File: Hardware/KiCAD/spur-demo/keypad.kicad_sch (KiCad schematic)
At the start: 40 parts, among them SW10 *, SW11 4, SW12 5, SW13 6, SW14 0, SW15 7, SW16 8, SW17 9, SW18 #, SW19 PTT, SW20 LEFT, SW21 RIGHT, SW22 SK0, SW3 MENU, SW4 UP, SW5 DOWN, SW6 EXIT, SW7 1, SW8 2, SW9 3

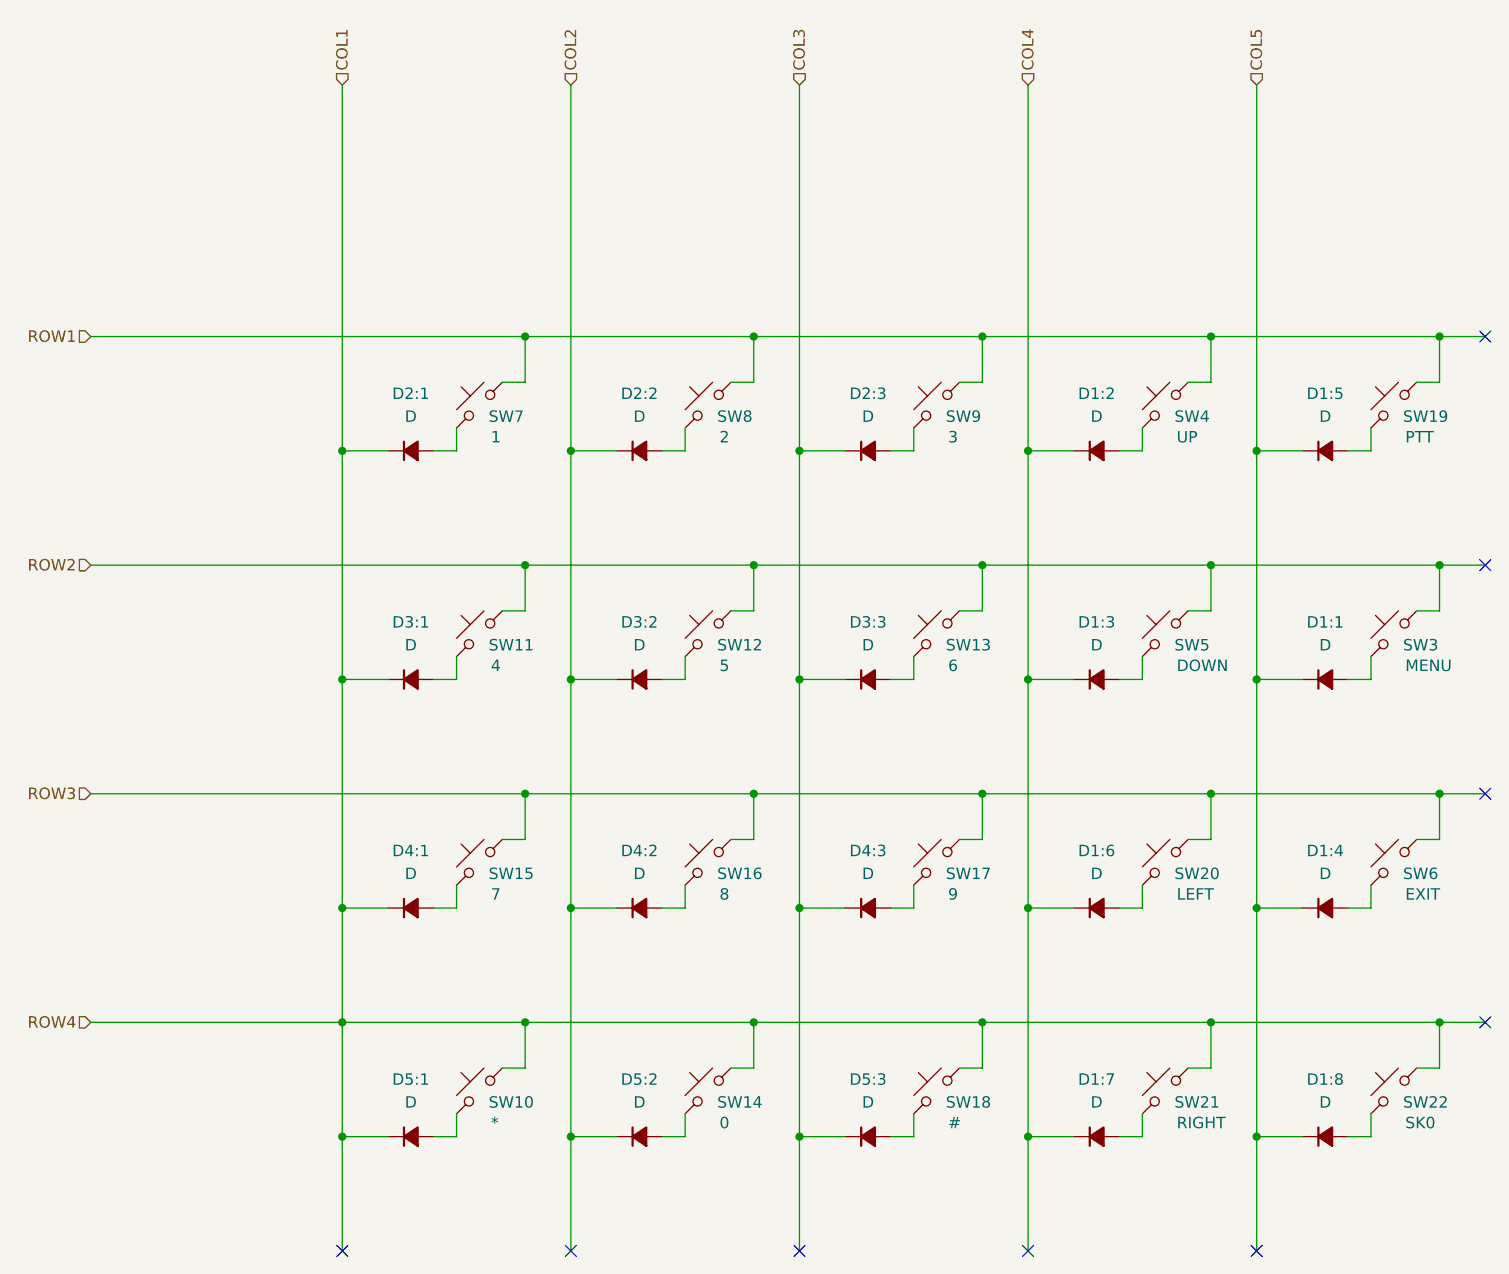
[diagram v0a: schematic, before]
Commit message: fix: remove node breaking col1 and row4 net resolution
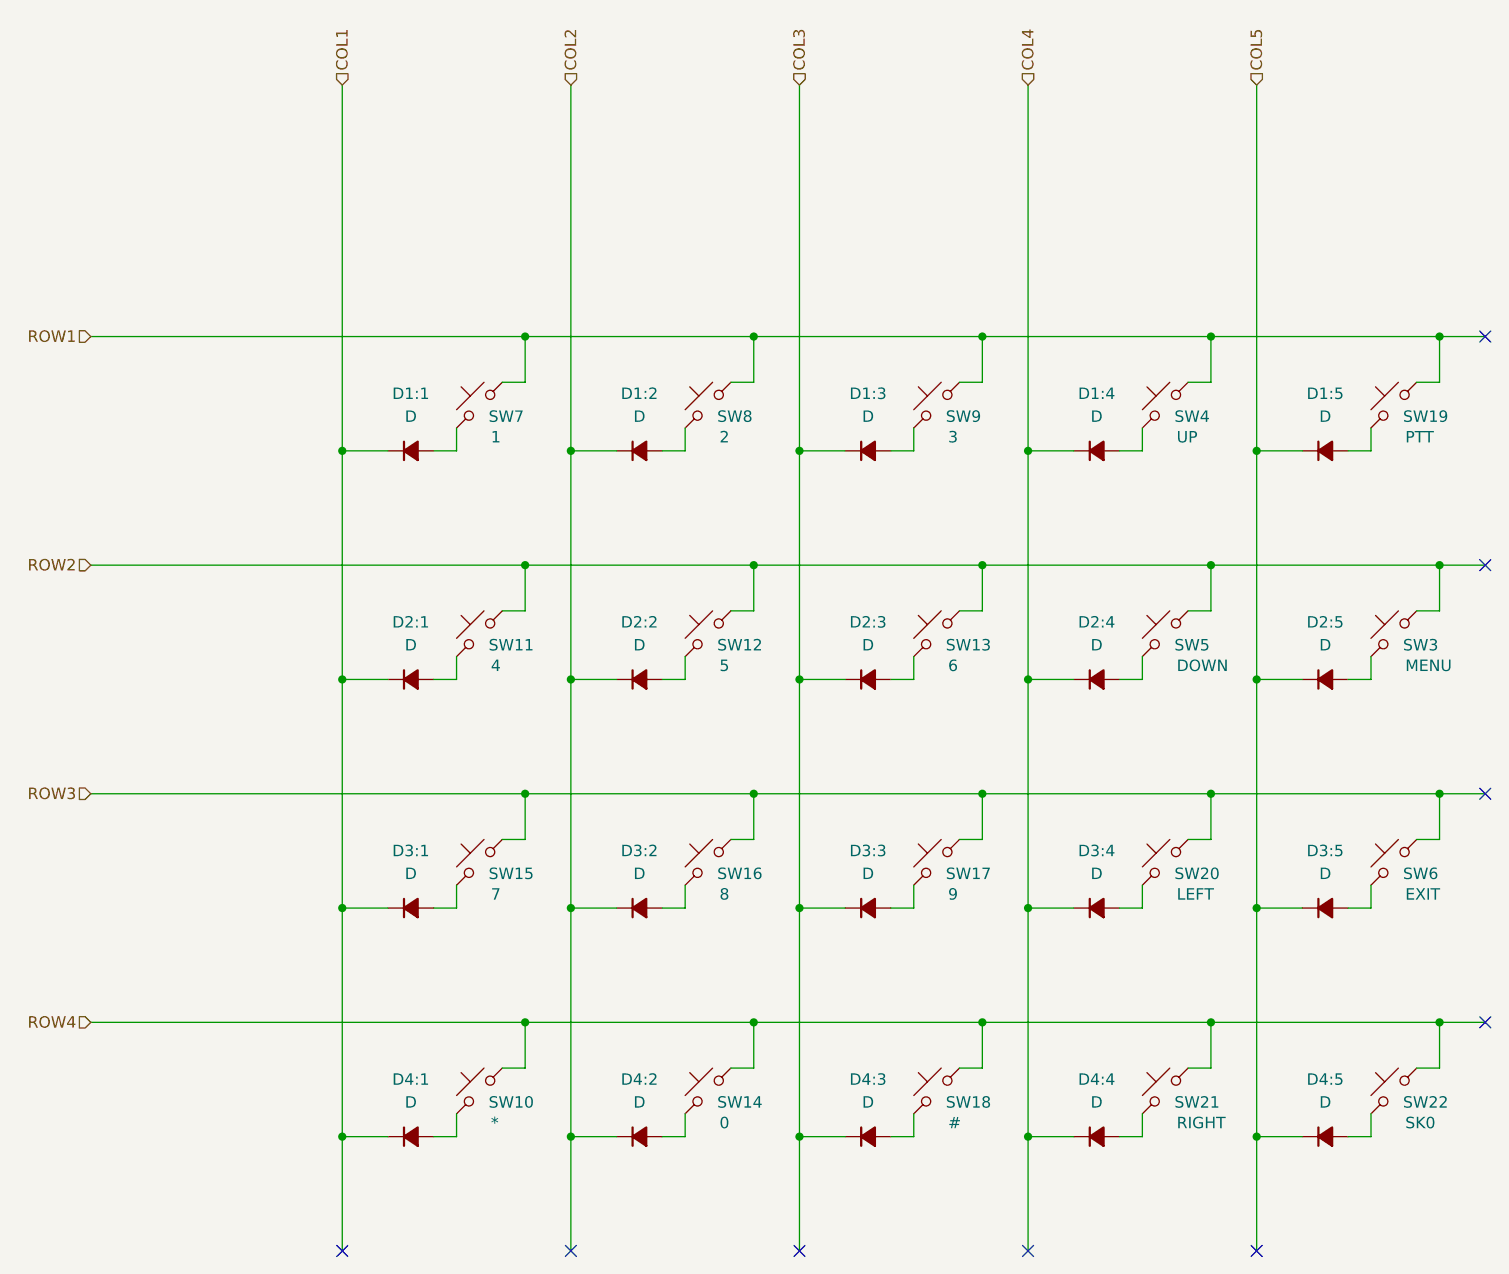
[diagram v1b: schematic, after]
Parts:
- renumbered D2:1 to D1:1, D2:2 to D1:2, D2:3 to D1:3, D1:2 to D1:4, D3:1 to D2:1, D3:2 to D2:2, D3:3 to D2:3, D1:3 to D2:4, D1:1 to D2:5, D4:1 to D3:1, D4:2 to D3:2, D4:3 to D3:3, D1:6 to D3:4, D1:4 to D3:5, D5:1 to D4:1, D5:2 to D4:2, D5:3 to D4:3, D1:7 to D4:4, D1:8 to D4:5
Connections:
- net COL1: no longer SW10.2, SW14.2, SW18.2, SW21.2, SW22.2
- new net ROW4: SW10.2, SW14.2, SW18.2, SW21.2, SW22.2
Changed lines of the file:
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@@
 	)
 	(junction
-		(at 76.2 135.89)
-		(diameter 0)
-		(color 0 0 0 0)
-	)
-	(junction
 		(at 127 123.19)
 		(diameter 0)
@@
 	(wire
 		(pts
-			(xy 76.2 123.19) (xy 76.2 135.89)
+			(xy 76.2 123.19) (xy 76.2 148.59)
 		)
 		(stroke
@@
 	(wire
 		(pts
-			(xy 48.26 135.89) (xy 76.2 135.89)
+			(xy 48.26 135.89) (xy 96.52 135.89)
 		)
 		(stroke
@@
 	(wire
 		(pts
-			(xy 76.2 135.89) (xy 76.2 148.59)
-		)
-		(stroke
-			(width 0)
-			(type default)
-		)
-	)
-	(wire
-		(pts
 			(xy 152.4 97.79) (xy 157.48 97.79)
 		)
@@
 	(wire
 		(pts
-			(xy 76.2 135.89) (xy 96.52 135.89)
-		)
-		(stroke
-			(width 0)
-			(type default)
-		)
-	)
-	(wire
-		(pts
 			(xy 93.98 140.97) (xy 96.52 140.97)
 		)
@@
 		(dnp no)
 		(fields_autoplaced yes)
-		(property "Reference" "D4:1"
+		(property "Reference" "D3:1"
 			(at 83.82 116.84 0)
 			(effects
@@
 			(project "spur-demo"
 				(path "/48a1a14a-bba3-4ee0-af51-70720bbf1fda/e48efb72-302e-45b5-b9fb-6ddbb8e8c1ba"
-					(reference "D4:1")
+					(reference "D3:1")
 					(unit 1)
 				)
@@
 		(dnp no)
 		(fields_autoplaced yes)
-		(property "Reference" "D1:1"
+		(property "Reference" "D2:5"
 			(at 185.42 91.44 0)
 			(effects
@@
 			(project "spur-demo"
 				(path "/48a1a14a-bba3-4ee0-af51-70720bbf1fda/e48efb72-302e-45b5-b9fb-6ddbb8e8c1ba"
-					(reference "D1:1")
+					(reference "D2:5")
 					(unit 1)
 				)
@@
 		(dnp no)
 		(fields_autoplaced yes)
-		(property "Reference" "D3:1"
+		(property "Reference" "D2:1"
 			(at 83.82 91.44 0)
 			(effects
@@
 			(project "spur-demo"
 				(path "/48a1a14a-bba3-4ee0-af51-70720bbf1fda/e48efb72-302e-45b5-b9fb-6ddbb8e8c1ba"
-					(reference "D3:1")
+					(reference "D2:1")
 					(unit 1)
 				)
@@
 		(dnp no)
 		(fields_autoplaced yes)
-		(property "Reference" "D2:3"
+		(property "Reference" "D1:3"
 			(at 134.62 66.04 0)
 			(effects
@@
 			(project "spur-demo"
 				(path "/48a1a14a-bba3-4ee0-af51-70720bbf1fda/e48efb72-302e-45b5-b9fb-6ddbb8e8c1ba"
-					(reference "D2:3")
+					(reference "D1:3")
 					(unit 1)
 				)
@@
 		(dnp no)
 		(fields_autoplaced yes)
-		(property "Reference" "D1:2"
+		(property "Reference" "D1:4"
 			(at 160.02 66.04 0)
 			(effects
@@
 			(project "spur-demo"
 				(path "/48a1a14a-bba3-4ee0-af51-70720bbf1fda/e48efb72-302e-45b5-b9fb-6ddbb8e8c1ba"
-					(reference "D1:2")
+					(reference "D1:4")
 					(unit 1)
 				)
@@
 		(dnp no)
 		(fields_autoplaced yes)
-		(property "Reference" "D5:3"
+		(property "Reference" "D4:3"
 			(at 134.62 142.24 0)
 			(effects
@@
 			(project "spur-demo"
 				(path "/48a1a14a-bba3-4ee0-af51-70720bbf1fda/e48efb72-302e-45b5-b9fb-6ddbb8e8c1ba"
-					(reference "D5:3")
+					(reference "D4:3")
 					(unit 1)
 				)
@@
 		(dnp no)
 		(fields_autoplaced yes)
-		(property "Reference" "D2:1"
+		(property "Reference" "D1:1"
 			(at 83.82 66.04 0)
 			(effects
@@
 			(project "spur-demo"
 				(path "/48a1a14a-bba3-4ee0-af51-70720bbf1fda/e48efb72-302e-45b5-b9fb-6ddbb8e8c1ba"
-					(reference "D2:1")
+					(reference "D1:1")
 					(unit 1)
 				)
@@
 		(dnp no)
 		(fields_autoplaced yes)
-		(property "Reference" "D3:2"
+		(property "Reference" "D2:2"
 			(at 109.22 91.44 0)
 			(effects
@@
 			(project "spur-demo"
 				(path "/48a1a14a-bba3-4ee0-af51-70720bbf1fda/e48efb72-302e-45b5-b9fb-6ddbb8e8c1ba"
-					(reference "D3:2")
+					(reference "D2:2")
 					(unit 1)
 				)
@@
 		(dnp no)
 		(fields_autoplaced yes)
-		(property "Reference" "D1:3"
+		(property "Reference" "D2:4"
 			(at 160.02 91.44 0)
 			(effects
@@
 			(project "spur-demo"
 				(path "/48a1a14a-bba3-4ee0-af51-70720bbf1fda/e48efb72-302e-45b5-b9fb-6ddbb8e8c1ba"
-					(reference "D1:3")
+					(reference "D2:4")
 					(unit 1)
 				)
@@
 		(dnp no)
 		(fields_autoplaced yes)
-		(property "Reference" "D4:3"
+		(property "Reference" "D3:3"
 			(at 134.62 116.84 0)
 			(effects
@@
 			(project "spur-demo"
 				(path "/48a1a14a-bba3-4ee0-af51-70720bbf1fda/e48efb72-302e-45b5-b9fb-6ddbb8e8c1ba"
-					(reference "D4:3")
+					(reference "D3:3")
 					(unit 1)
 				)
@@
 		(dnp no)
 		(fields_autoplaced yes)
-		(property "Reference" "D3:3"
+		(property "Reference" "D2:3"
 			(at 134.62 91.44 0)
 			(effects
@@
 			(project "spur-demo"
 				(path "/48a1a14a-bba3-4ee0-af51-70720bbf1fda/e48efb72-302e-45b5-b9fb-6ddbb8e8c1ba"
-					(reference "D3:3")
+					(reference "D2:3")
 					(unit 1)
 				)
@@
 		(dnp no)
 		(fields_autoplaced yes)
-		(property "Reference" "D1:4"
+		(property "Reference" "D3:5"
 			(at 185.42 116.84 0)
 			(effects
@@
 			(project "spur-demo"
 				(path "/48a1a14a-bba3-4ee0-af51-70720bbf1fda/e48efb72-302e-45b5-b9fb-6ddbb8e8c1ba"
-					(reference "D1:4")
+					(reference "D3:5")
 					(unit 1)
 				)
@@
 		(dnp no)
 		(fields_autoplaced yes)
-		(property "Reference" "D1:8"
+		(property "Reference" "D4:5"
 			(at 185.42 142.24 0)
 			(effects
@@
 			(project "spur-demo"
 				(path "/48a1a14a-bba3-4ee0-af51-70720bbf1fda/e48efb72-302e-45b5-b9fb-6ddbb8e8c1ba"
-					(reference "D1:8")
+					(reference "D4:5")
 					(unit 1)
 				)
@@
 		(dnp no)
 		(fields_autoplaced yes)
-		(property "Reference" "D4:2"
+		(property "Reference" "D3:2"
 			(at 109.22 116.84 0)
 			(effects
@@
 			(project "spur-demo"
 				(path "/48a1a14a-bba3-4ee0-af51-70720bbf1fda/e48efb72-302e-45b5-b9fb-6ddbb8e8c1ba"
-					(reference "D4:2")
+					(reference "D3:2")
 					(unit 1)
 				)
@@
 		(dnp no)
 		(fields_autoplaced yes)
-		(property "Reference" "D1:7"
+		(property "Reference" "D4:4"
 			(at 160.02 142.24 0)
 			(effects
@@
 			(project "spur-demo"
 				(path "/48a1a14a-bba3-4ee0-af51-70720bbf1fda/e48efb72-302e-45b5-b9fb-6ddbb8e8c1ba"
-					(reference "D1:7")
+					(reference "D4:4")
 					(unit 1)
 				)
@@
 		(dnp no)
 		(fields_autoplaced yes)
-		(property "Reference" "D1:6"
+		(property "Reference" "D3:4"
 			(at 160.02 116.84 0)
 			(effects
@@
 			(project "spur-demo"
 				(path "/48a1a14a-bba3-4ee0-af51-70720bbf1fda/e48efb72-302e-45b5-b9fb-6ddbb8e8c1ba"
-					(reference "D1:6")
+					(reference "D3:4")
 					(unit 1)
 				)
@@
 		(dnp no)
 		(fields_autoplaced yes)
-		(property "Reference" "D2:2"
+		(property "Reference" "D1:2"
 			(at 109.22 66.04 0)
 			(effects
@@
 			(project "spur-demo"
 				(path "/48a1a14a-bba3-4ee0-af51-70720bbf1fda/e48efb72-302e-45b5-b9fb-6ddbb8e8c1ba"
-					(reference "D2:2")
+					(reference "D1:2")
 					(unit 1)
 				)
@@
 		(dnp no)
 		(fields_autoplaced yes)
-		(property "Reference" "D5:1"
+		(property "Reference" "D4:1"
 			(at 83.82 142.24 0)
 			(effects
@@
 			(project "spur-demo"
 				(path "/48a1a14a-bba3-4ee0-af51-70720bbf1fda/e48efb72-302e-45b5-b9fb-6ddbb8e8c1ba"
-					(reference "D5:1")
+					(reference "D4:1")
 					(unit 1)
 				)
@@
 		(dnp no)
 		(fields_autoplaced yes)
-		(property "Reference" "D5:2"
+		(property "Reference" "D4:2"
 			(at 109.22 142.24 0)
 			(effects
@@
 			(project "spur-demo"
 				(path "/48a1a14a-bba3-4ee0-af51-70720bbf1fda/e48efb72-302e-45b5-b9fb-6ddbb8e8c1ba"
-					(reference "D5:2")
+					(reference "D4:2")
 					(unit 1)
 				)
